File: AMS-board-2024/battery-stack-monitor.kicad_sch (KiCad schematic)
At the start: 71 parts, among them Q115 STD7ANM60N, Q116 2N7002K-AU, Q117 STD7ANM60N, Q118 STD7ANM60N, U23 LM25180-Q1, U24 NCV8711BMTW500TBG, U25 LTC2949, U26 NV24C16SNVLT3G, Y2 ABLS-4.000MHZ-K4T

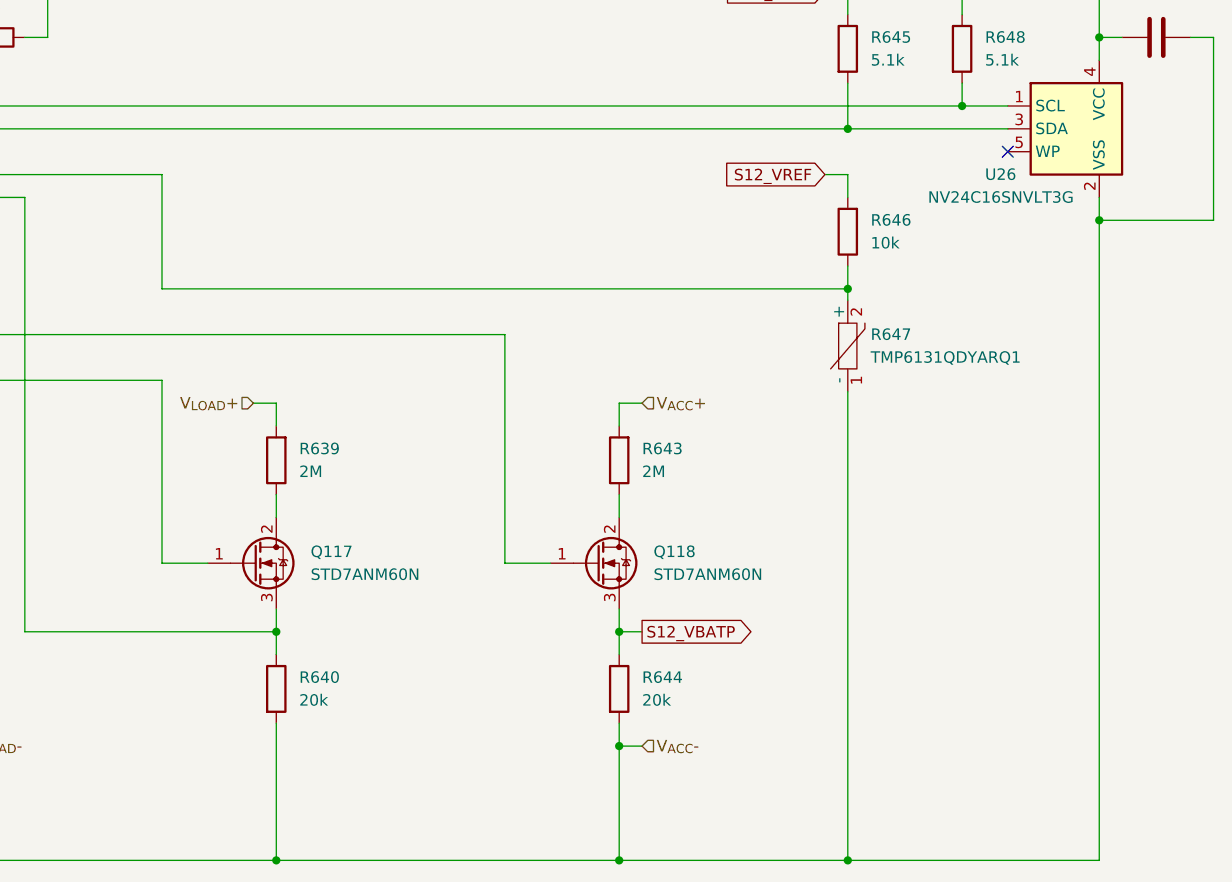
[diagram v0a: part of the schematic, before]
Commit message: サーミスタのマイナス側をシャント抵抗に接続
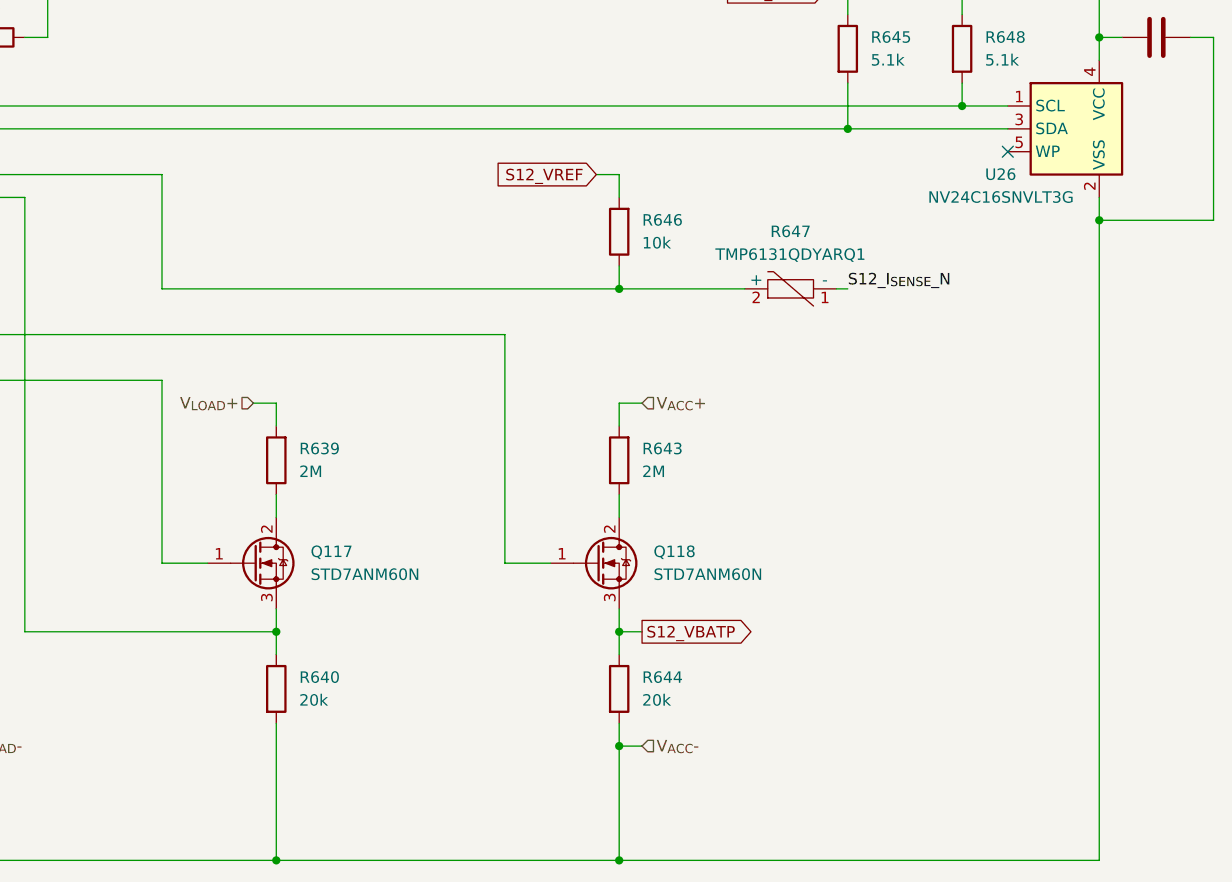
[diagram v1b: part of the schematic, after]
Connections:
- net S12_I_{SENSE}_N: now also R647.1 (-)
- net V_{ACC}-: no longer R647.1 (-)
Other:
- moved on the sheet: R646, R647
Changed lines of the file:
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@@
   (junction (at 165.1 167.64) (diameter 0) (color 0 0 0 0)
   )
-  (junction (at 355.6 241.3) (diameter 0) (color 0 0 0 0)
-  )
   (junction (at 177.8 142.24) (diameter 0) (color 0 0 0 0)
   )
@@
   (junction (at 218.44 109.22) (diameter 0) (color 0 0 0 0)
   )
-  (junction (at 355.6 177.8) (diameter 0) (color 0 0 0 0)
+  (junction (at 330.2 177.8) (diameter 0) (color 0 0 0 0)
   )
   (junction (at 203.2 200.66) (diameter 0) (color 0 0 0 0)
@@
     (stroke (width 0) (type default))
   )
-  (wire (pts (xy 383.54 241.3) (xy 355.6 241.3))
+  (wire (pts (xy 330.2 241.3) (xy 383.54 241.3))
     (stroke (width 0) (type default))
   )
@@
     (stroke (width 0) (type default))
   )
-  (wire (pts (xy 353.06 165.1) (xy 355.6 165.1))
+  (wire (pts (xy 327.66 165.1) (xy 330.2 165.1))
     (stroke (width 0) (type default))
   )
@@
     (stroke (width 0) (type default))
   )
-  (wire (pts (xy 330.2 241.3) (xy 355.6 241.3))
-    (stroke (width 0) (type default))
-  )
   (wire (pts (xy 165.1 167.64) (xy 167.64 167.64))
     (stroke (width 0) (type default))
@@
     (stroke (width 0) (type default))
   )
-  (wire (pts (xy 355.6 177.8) (xy 279.4 177.8))
+  (wire (pts (xy 330.2 177.8) (xy 279.4 177.8))
     (stroke (width 0) (type default))
   )
@@
     (stroke (width 0) (type default))
   )
-  (wire (pts (xy 355.6 189.23) (xy 355.6 241.3))
-    (stroke (width 0) (type default))
-  )
   (wire (pts (xy 292.1 190.5) (xy 292.1 193.04))
     (stroke (width 0) (type default))
@@
     (stroke (width 0) (type default))
   )
+  (wire (pts (xy 354.33 177.8) (xy 355.6 177.8))
+    (stroke (width 0) (type default))
+  )
   (wire (pts (xy 177.8 152.4) (xy 177.8 160.02))
     (stroke (width 0) (type default))
@@
     (stroke (width 0) (type default))
   )
-  (wire (pts (xy 355.6 175.26) (xy 355.6 177.8))
+  (wire (pts (xy 330.2 175.26) (xy 330.2 177.8))
     (stroke (width 0) (type default))
   )
@@
     (stroke (width 0) (type default))
   )
-  (wire (pts (xy 355.6 177.8) (xy 355.6 179.07))
-    (stroke (width 0) (type default))
-  )
   (wire (pts (xy 198.12 91.44) (xy 198.12 93.98))
     (stroke (width 0) (type default))
   )
+  (wire (pts (xy 330.2 177.8) (xy 344.17 177.8))
+    (stroke (width 0) (type default))
+  )
   (wire (pts (xy 205.74 198.12) (xy 205.74 200.66))
     (stroke (width 0) (type default))
@@
     (stroke (width 0) (type default))
   )
-  (wire (pts (xy 355.6 165.1) (xy 355.6 167.64))
+  (wire (pts (xy 330.2 165.1) (xy 330.2 167.64))
     (stroke (width 0) (type default))
   )
@@
     (effects (font (size 1.27 1.27)) (justify left bottom))
   )
-  (global_label "S12_VREF" (shape input) (at 353.06 165.1 180) (fields_autoplaced)
+  (label "S12_I_{SENSE}_N" (at 355.6 177.8 0) (fields_autoplaced)
+    (effects (font (size 1.27 1.27)) (justify left bottom))
+  )
+  (global_label "S12_VREF" (shape input) (at 327.66 165.1 180) (fields_autoplaced)
     (effects (font (size 1.27 1.27)) (justify right))
-    (property "Intersheetrefs" "${INTERSHEET_REFS}" (at 340.8825 165.1 0)
+    (property "Intersheetrefs" "${INTERSHEET_REFS}" (at 315.4825 165.1 0)
       (effects (font (size 1.27 1.27)) (justify right) hide)
     )
@@
     )
   )
-  (symbol (lib_id "Device:R") (at 355.6 171.45 180) (unit 1)
-    (in_bom yes) (on_board yes) (dnp no) (fields_autoplaced)
-    (property "Reference" "R646" (at 358.14 170.18 0)
+  (symbol (lib_id "Device:R") (at 330.2 171.45 180) (unit 1)
+    (in_bom yes) (on_board yes) (dnp no) (fields_autoplaced)
+    (property "Reference" "R646" (at 332.74 170.18 0)
       (effects (font (size 1.27 1.27)) (justify right))
     )
-    (property "Value" "10k" (at 358.14 172.72 0)
+    (property "Value" "10k" (at 332.74 172.72 0)
       (effects (font (size 1.27 1.27)) (justify right))
     )
-    (property "Footprint" "Resistor_SMD:R_0402_1005Metric" (at 357.378 171.45 90)
-      (effects (font (size 1.27 1.27)) hide)
-    )
-    (property "Datasheet" "~" (at 355.6 171.45 0)
+    (property "Footprint" "Resistor_SMD:R_0402_1005Metric" (at 331.978 171.45 90)
+      (effects (font (size 1.27 1.27)) hide)
+    )
+    (property "Datasheet" "~" (at 330.2 171.45 0)
       (effects (font (size 1.27 1.27)) hide)
     )
@@
     )
   )
-  (symbol (lib_id "ProjectEV:Sensor_TMP6131QDYARQ1") (at 355.6 184.15 0) (unit 1)
-    (in_bom yes) (on_board yes) (dnp no) (fields_autoplaced)
-    (property "Reference" "R647" (at 358.14 182.88 0)
-      (effects (font (size 1.27 1.27)) (justify left))
-    )
-    (property "Value" "TMP6131QDYARQ1" (at 358.14 185.42 0)
-      (effects (font (size 1.27 1.27)) (justify left))
-    )
-    (property "Footprint" "ProjectEV:Package_SOD-523_TMP6131QDYARQ1" (at 355.6 184.15 0)
-      (effects (font (size 1.27 1.27)) hide)
-    )
-    (property "Datasheet" "https://www.ti.com/lit/ds/symlink/tmp61-q1.pdf" (at 355.6 195.58 0)
-      (effects (font (size 1.27 1.27)) hide)
-    )
+  (symbol (lib_id "ProjectEV:Sensor_TMP6131QDYARQ1") (at 349.25 177.8 90) (unit 1)
+    (in_bom yes) (on_board yes) (dnp no) (fields_autoplaced)
+    (property "Reference" "R647" (at 349.25 171.45 90)
+      (effects (font (size 1.27 1.27)))
+    )
+    (property "Value" "TMP6131QDYARQ1" (at 349.25 173.99 90)
+      (effects (font (size 1.27 1.27)))
+    )
+    (property "Footprint" "ProjectEV:Package_SOD-523_TMP6131QDYARQ1" (at 349.25 177.8 0)
+      (effects (font (size 1.27 1.27)) hide)
+    )
+    (property "Datasheet" "https://www.ti.com/lit/ds/symlink/tmp61-q1.pdf" (at 360.68 177.8 0)
+      (effects (font (size 1.27 1.27)) hide)
+    )
